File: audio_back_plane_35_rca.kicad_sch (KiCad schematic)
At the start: 55 parts, among them J2 SJ3-35044A, J4 Conn_01x10, J5 Conn_02x10_Odd_Even, J6 SJ3-35044A, SW1 SW_SPST, SW2 SW_SPST, SW3 SW1, U1 ESP32-DevKitC - DEVKIT, U3 Teensy 4.1 - DEVKIT

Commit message: update
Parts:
- removed BYPASS1: jumper, project_fp:SolderJumper-2_P1.3mm_Bridged2Bar_RoundedPad1.0x1.5mm_OPEN, symbol Jumper:SolderJumper_2_Open
- removed EPROG1: header, project_fp:EPROG1_PinHeader_1x06_P2.54mm_Vertical, symbol Connector_Generic:Conn_01x06
- removed ESP_I1: header, project_fp:ESP_I2C_0_PinHeader_2x02_P2.54mm_Vertical, symbol Connector_Generic:Conn_02x02_Odd_Even
- removed GPI1: header, project_fp:GPI1_PinHeader_1x04_P2.54mm_Vertical, symbol Connector_Generic:Conn_01x04
- removed ILI1: ILI9341+XPT2046, project_fp:ILI9341_PinHeader_1x14_P2.54mm_Vertical, symbol project_lil_2:ILI9341_header
- removed ILI_VCC1: jumper, project_fp:SolderJumper-3_P1.3mm_Bridged2Bar12_Pad1.0x1.5mm_NumberLabels, symbol Jumper:SolderJumper_3_Bridged12
- removed J2, J6: SJ3-35044A, project_fp:SAMESKY_SJ3-35044A, symbol SJ3-35044A:SJ3-35044A
- removed J4: Conn_01x10, Connector_PinHeader_2.54mm:PinHeader_1x10_P2.54mm_Vertical, symbol Connector_Generic:Conn_01x10
- removed J5: Conn_02x10_Odd_Even, Connector_IDC:IDC-Header_2x10_P2.54mm_Vertical, symbol Connector_Generic:Conn_02x10_Odd_Even
- removed R15, R2, R3, R4, R5: 2.2k ohm - 2200 ohm, Resistor_THT:R_Axial_DIN0204_L3.6mm_D1.6mm_P5.08mm_Horizontal, symbol Device:R
- removed SW1, SW2: SW_SPST, project_fp:SW_Tactile_SPST_Angled_PTS645Vx39-2LFS, symbol Switch:SW_SPST
- removed USB_HOST1: header, project_fp:USB_OUT1, symbol project_lil_2:USB_header_1x5_2.54
- added D3, D4: SK6812_4020_SIDE_LED, project_fp:LED_4691, symbol SK6812_4020_SIDE_LED:SK6812_4020_SIDE_LED
- D1, D2: value WS2812B - COM-16347 -> HEADER; footprint Connector_PinHeader_1.00mm:PinHeader_1x04_P1.00mm_Vertical -> project_fp:PinHeader_1x04_P1.00mm_Vertical_WS2812_LED_mod; now not fitted
- G1, HPTRS1, HPTRS2, U1, U3, board_outline2: now not fitted
- R1, R10, R12, R13, R14, R17, R19, R20, R21, R6, R7, R8, R9: footprint Resistor_THT:R_Axial_DIN0204_L3.6mm_D1.6mm_P5.08mm_Horizontal -> project_fp:R_0805_2012Metric_Pad1.20x1.40mm_HandSolder
- SW3: value SW1 -> OS102011MA1QN1
- board_outline1: value board -> TAC5212 Module; now not fitted
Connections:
- net 3.3V: now also MIC2.2 (SELECT)
- net 34_RX8_RESET2: no longer U3.26 (34_RX8)
- net 5V: now also D3.2 (VDD), D4.2 (VDD)
- net GND: now also MIC1.2 (SELECT), D3.4 (GND), D4.4 (GND)
- net at SW3.2 (C): now also HPTRS2.2; no longer HPTRS2.5
- net at board_outline1.21 (OUTP): now also HPTRS1.5; no longer HPTRS1.2
- net at board_outline1.25 (OUT2P): now also HPTRS1.2; no longer HPTRS1.5
- net at board_outline1.29 (IN1P): now also HPTRS2.5; no longer HPTRS2.2
- net at D2.1 (Pin_1), R17.1: now also D4.1 (DIN)
- net at D1.1 (Pin_1), R13.1: now also D3.1 (DIN)
- net ESP32_IO21_SDA: no longer names the net of U1.33 (GPIO21)
- net ESP32_IO22_SCL: no longer names the net of U1.36 (GPIO22)
- net MIDI_RX: no longer names the net of U3.2 (0_RX1_CRX2_CS1)
- net MIDI_TX_T: no longer names the net of U3.3 (1_TX1_CTX2_MISO1)
- net T_BUTTON1: no longer names the net of U3.16 (24_A10_TX6_SCL2)
- net T_BUTTON2: no longer names the net of U3.17 (25_A11_RX6_SDA2)
- new net: MIC1.4 (LRCLK-WS-FS), MIC2.4 (LRCLK-WS-FS), board_outline1.40 (GPIO1)
- now unconnected: MIC1.4 (LRCLK-WS-FS), MIC2.4 (LRCLK-WS-FS)
- no-connect marks 8 -> 6
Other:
- moved on the sheet: C8, R13, R17, SW3, USBA1

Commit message: update
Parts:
- added D10, D11, D5, D6, D7, D8: SK6812, project_fp:LED_SK6812_EC15_1.5x1.5mm, symbol SK6812_4020_SIDE_LED:SK6812_REVERSE_MOUNT
- added D9: SK6812, project_fp:LED_SK6812, symbol SK6812:SK6812
- added SW1: RotaryEncoder_Switch_MP, project_fp:RotaryEncoder_Alps_EC11E_Vertical_H20mm, symbol Device:RotaryEncoder_Switch_MP
- added SW2, SW4, SW5, SW6: TL1105WF160Q - 3.15mm actuator, project_fp:Tactile_Switch_4.54.5MM, symbol Switch:SW_SPST
- D3, D4: value SK6812_4020_SIDE_LED -> SK6812; footprint project_fp:LED_4691 -> project_fp:LED_SK6812_EC15_1.5x1.5mm; symbol SK6812_4020_SIDE_LED:SK6812_4020_SIDE_LED -> SK6812_4020_SIDE_LED:SK6812_REVERSE_MOUNT
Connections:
- net 5V: now also D3.1 (VDD), D4.1 (VDD), D5.1 (VDD), D6.1 (VDD); no longer D3.2 (VDD), D4.2 (VDD)
- net GND: now also D3.3 (GND), D4.3 (GND), D5.3 (GND); no longer D3.4 (GND), D4.4 (GND)
- net at D2.1 (Pin_1), R17.1: now also D4.4 (DIN); no longer D4.1 (DIN)
- net at D1.1 (Pin_1), R13.1: now also D3.4 (DIN); no longer D3.1 (DIN)
- net T_BUTTON1: now reaches U3.16 (24_A10_TX6_SCL2)
- net T_BUTTON1: now also SW2.1 (A), SW5.1 (A)
- net T_BUTTON2: now reaches U3.17 (25_A11_RX6_SDA2)
- net T_BUTTON2: now also SW4.1 (A), SW6.1 (A)
- new net: MIC1.4 (LRCLK-WS-FS), MIC2.4 (LRCLK-WS-FS), board_outline1.40 (GPIO1)
- new net: D4.2 (DOUT), D5.4 (DIN)
- new net: D3.2 (DOUT), D6.4 (DIN)
- now unconnected: MIC1.4 (LRCLK-WS-FS), MIC2.4 (LRCLK-WS-FS)
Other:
- note added: "SWITCHES"

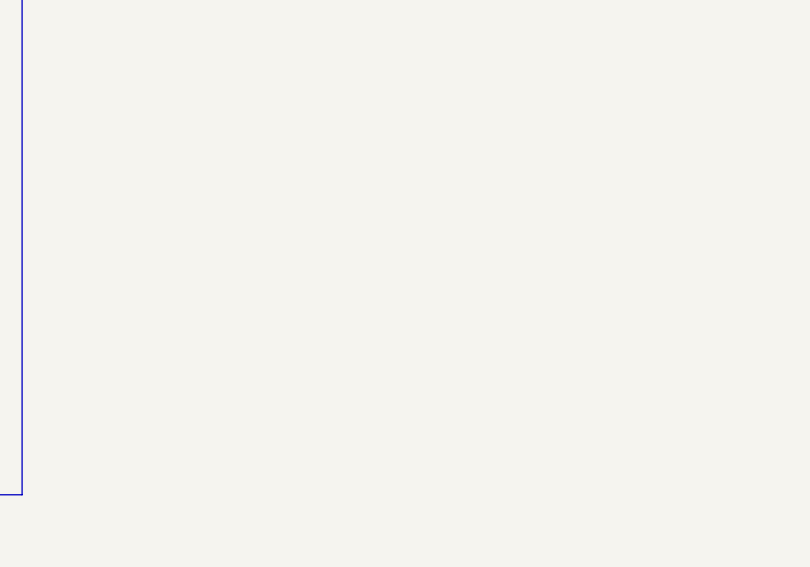
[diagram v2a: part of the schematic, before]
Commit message: update
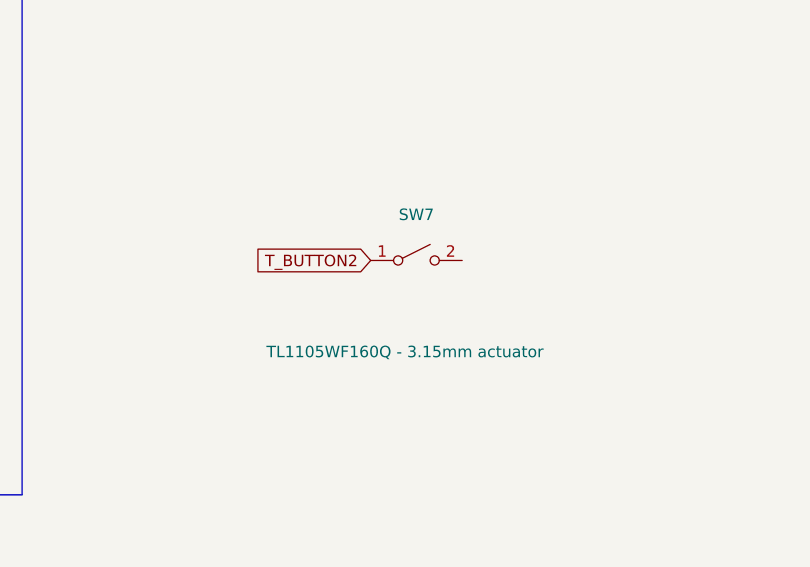
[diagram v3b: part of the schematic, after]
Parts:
- added SW7: TL1105WF160Q - 3.15mm actuator, project_fp:Tactile_Switch_4.54.5MM, symbol Switch:SW_SPST
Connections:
- net T_BUTTON2: now also SW7.1 (A)
- new net: MIC1.4 (LRCLK-WS-FS), MIC2.4 (LRCLK-WS-FS), board_outline1.40 (GPIO1)
- now unconnected: MIC1.4 (LRCLK-WS-FS), MIC2.4 (LRCLK-WS-FS)
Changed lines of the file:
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@@
 		)
 	)
+	(global_label "T_BUTTON2"
+		(shape input)
+		(at 781.05 778.51 180)
+		(fields_autoplaced yes)
+		(effects
+			(font
+				(size 1.27 1.27)
+			)
+			(justify right)
+		)
+		(property "Intersheetrefs" "${INTERSHEET_REFS}"
+			(at 768.457 778.51 0)
+			(effects
+				(font
+					(size 1.27 1.27)
+				)
+				(justify right)
+				(hide yes)
+			)
+		)
+	)
 	(global_label "GND"
 		(shape input)
@@
 	)
 	(symbol
+		(lib_id "Switch:SW_SPST")
+		(at 786.13 778.51 0)
+		(unit 1)
+		(exclude_from_sim no)
+		(in_bom yes)
+		(on_board yes)
+		(dnp no)
+		(property "Reference" "SW7"
+			(at 786.13 773.43 0)
+			(effects
+				(font
+					(size 1.27 1.27)
+				)
+			)
+		)
+		(property "Value" "TL1105WF160Q - 3.15mm actuator"
+			(at 784.86 788.67 0)
+			(effects
+				(font
+					(size 1.27 1.27)
+				)
+			)
+		)
+		(property "Footprint" "project_fp:Tactile_Switch_4.54.5MM"
+			(at 786.13 778.51 0)
+			(effects
+				(font
+					(size 1.27 1.27)
+				)
+				(hide yes)
+			)
+		)
+		(property "Datasheet" "~"
+			(at 786.13 778.51 0)
+			(effects
+				(font
+					(size 1.27 1.27)
+				)
+				(hide yes)
+			)
+		)
+		(property "Description" ""
+			(at 786.13 778.51 0)
+			(effects
+				(font
+					(size 1.27 1.27)
+				)
+				(hide yes)
+			)
+		)
+		(pin "1"
+		)
+		(pin "2"
+		)
+		(instances
+			(project "audio_back_plane_35_rca"
+				(path "/6a0ff39d-771d-410f-9e7c-006586d81d16"
+					(reference "SW7")
+					(unit 1)
+				)
+			)
+		)
+	)
+	(symbol
 		(lib_id "power:GND")
 		(at 527.05 601.98 0)
@@
 	)
 	(symbol
-		(lib_name "lib_sch:SPH0645LM4H")
 		(lib_id "lib_sch:SPH0645LM4H")
 		(at 815.34 575.31 0)
@@
 	)
 	(symbol
-		(lib_name "lib_sch:SPH0645LM4H")
 		(lib_id "lib_sch:SPH0645LM4H")
 		(at 815.34 551.18 0)
